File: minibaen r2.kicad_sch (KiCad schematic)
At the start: 131 parts, among them J1 USB_C_Receptacle_USB2.0, Q1 2N7002, SW1 MX_SW_solder, SW10 MX_SW_solder, SW11 MX_SW_solder, SW12 MX_SW_solder, SW13 MX_SW_solder, SW14 MX_SW_solder, SW15 MX_SW_solder, SW16 MX_SW_solder, SW17 MX_SW_solder, SW18 MX_SW_solder, SW19 MX_SW_solder, SW2 MX_SW_solder, SW20 MX_SW_solder, SW21 MX_SW_solder, SW22 MX_SW_solder, SW23 MX_SW_solder, SW24 MX_SW_solder, SW25 MX_SW_solder, SW26 MX_SW_solder, SW27 MX_SW_solder, SW28 MX_SW_solder, SW29 MX_SW_solder, SW3 MX_SW_solder, SW30 MX_SW_solder, SW31 MX_SW_solder, SW32 MX_SW_solder, SW33 MX_SW_solder, SW34 MX_SW_solder, SW35 MX_SW_solder, SW36 MX_SW_solder, SW37 MX_SW_solder, SW38 MX_SW_solder, SW39 MX_SW_solder, SW4 MX_SW_solder, SW40 MX_SW_solder, SW41 MX_SW_solder, SW42 MX_SW_solder, SW43 MX_SW_solder, SW44 MX_SW_solder, SW45 MX_SW_solder, SW46 SW_Push, SW47 MX_SW_solder, SW48 MX_SW_solder, SW49 MX_SW_solder, SW5 MX_SW_solder, SW51 MX_SW_solder, SW52 MX_SW_solder, SW53 MX_SW_solder, SW54 MX_SW_solder, SW6 MX_SW_solder, SW7 MX_SW_solder, SW8 MX_SW_solder, SW9 MX_SW_solder, U3 SRV05-4, U4 XC6206PxxxMR, U5 STM32F072C8Tx

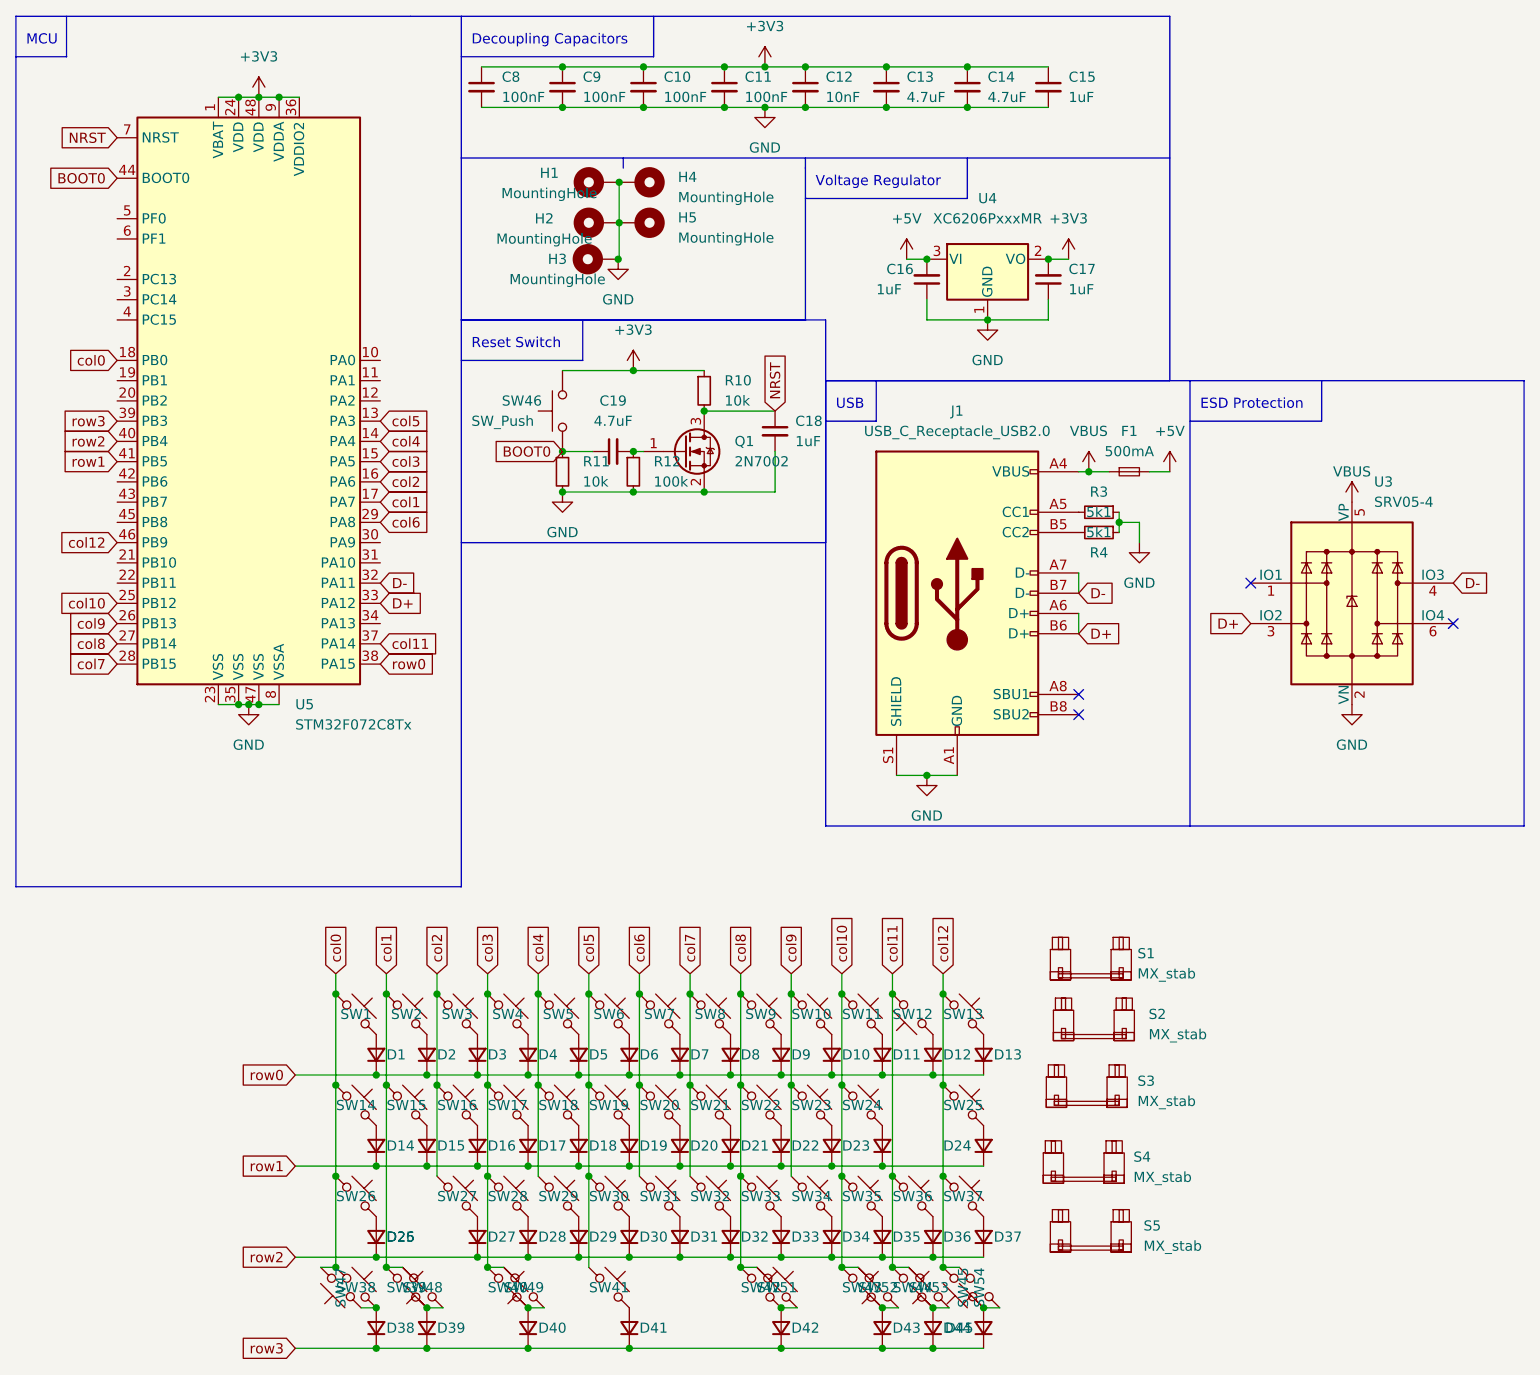
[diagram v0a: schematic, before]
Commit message: updates
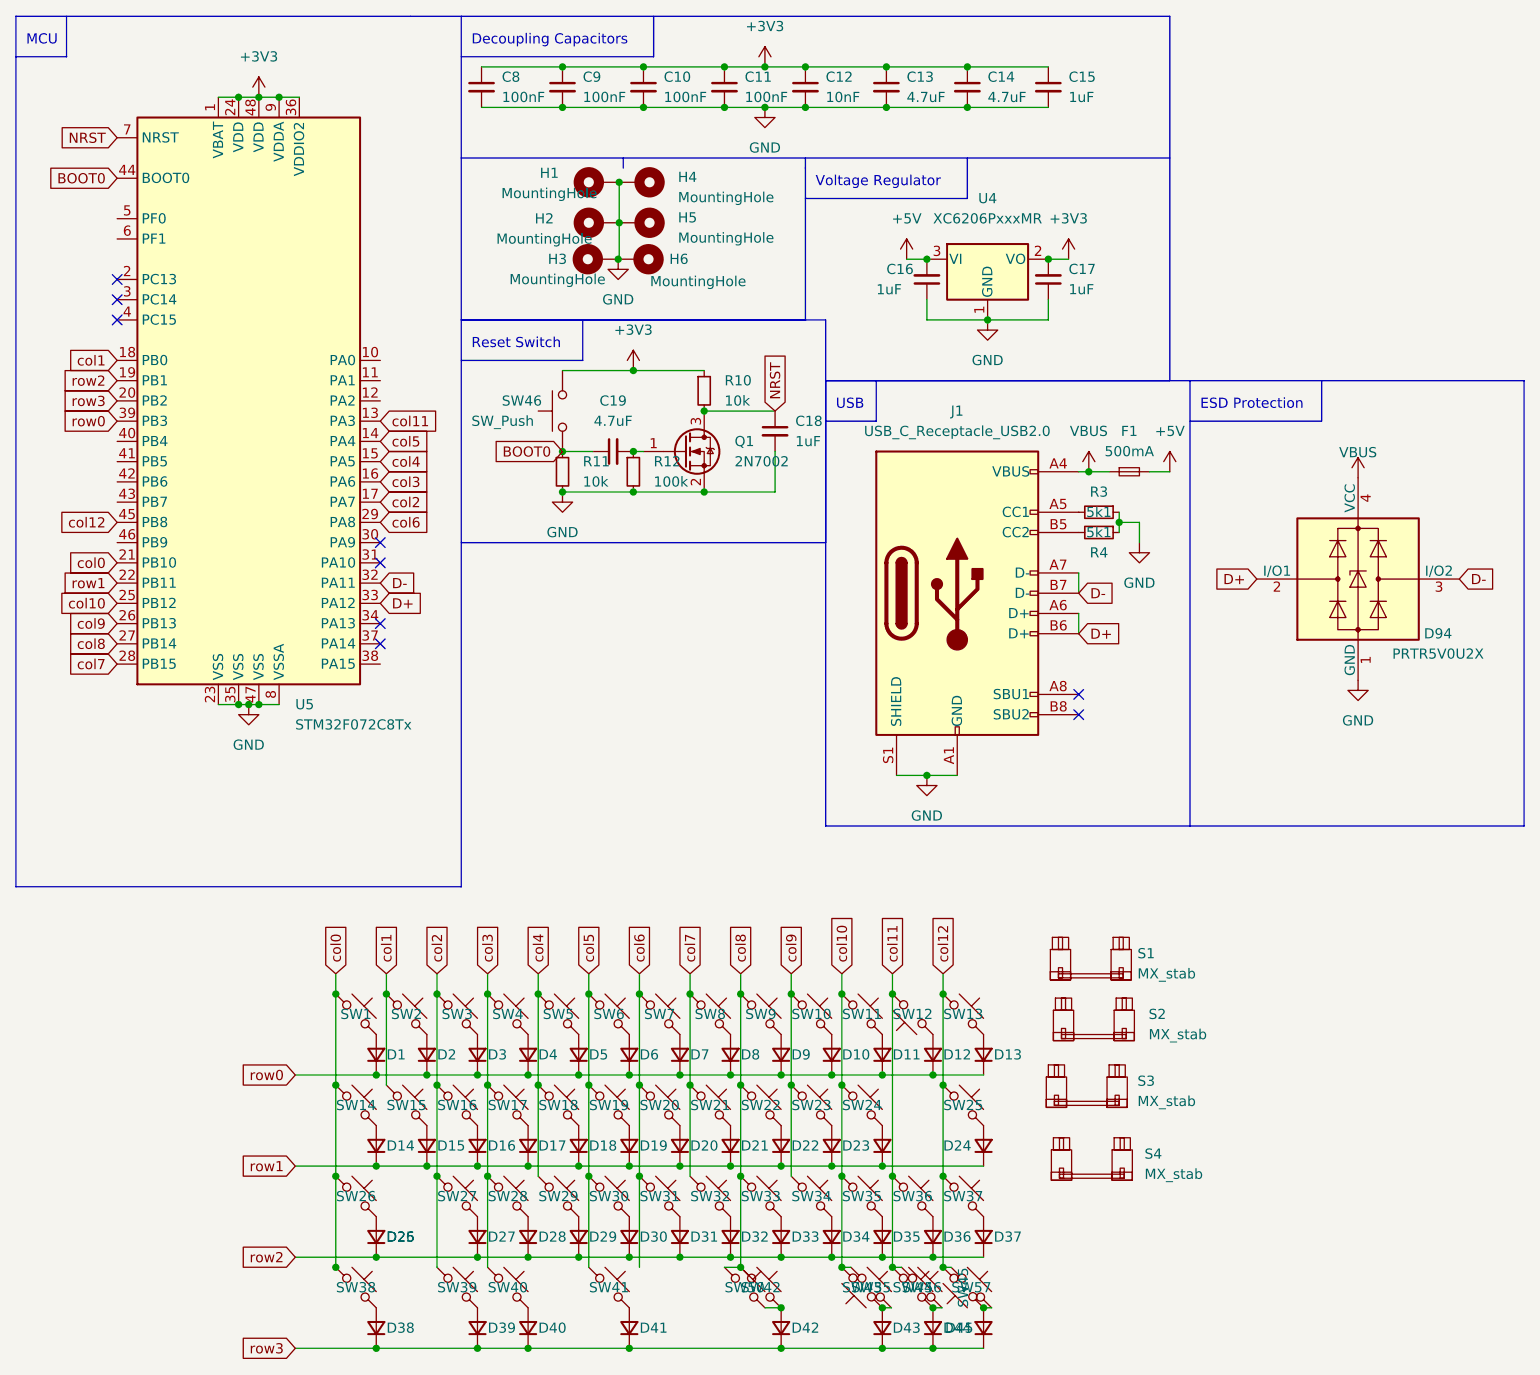
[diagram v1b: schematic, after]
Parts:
- removed S5: MX_stab, marbastlib-mx:STAB_MX_2u, symbol marbastlib-mx:MX_stab
- removed SW47, SW49, SW52, SW54: MX_SW_solder, marbastlib-mx:SW_MX_1.5u, symbol marbastlib-mx:MX_SW_solder
- removed SW48, SW51, SW53: MX_SW_solder, marbastlib-mx:SW_MX_1u, symbol marbastlib-mx:MX_SW_solder
- removed U3: SRV05-4, marbastlib-various:SOT-23-6-routable, symbol Power_Protection:SRV05-4
- added D94: PRTR5V0U2X, Package_TO_SOT_SMD:SOT-143, symbol Power_Protection:PRTR5V0U2X
- added H6: MountingHole, MountingHole:MountingHole_2.2mm_M2_DIN965_Pad, symbol Mechanical:MountingHole_Pad
- added SW50, SW55, SW56, SW57: MX_SW_solder, marbastlib-mx:SW_MX_1u, symbol marbastlib-mx:MX_SW_solder
- S4: footprint marbastlib-mx:STAB_MX_2.75u -> marbastlib-mx:STAB_MX_6.25u
- SW37: footprint marbastlib-mx:SW_MX_1.25u -> marbastlib-mx:SW_MX_1u
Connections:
- net D+: now also D94.2 (I/O1)
- net D-: now also D94.3 (I/O2)
- net GND: now also D94.1 (GND), H6.1
- net VBUS: now also D94.4 (VCC)
- net col0: now also U5.21 (PB10); no longer U5.18 (PB0)
- net col1: now also U5.18 (PB0); no longer SW39.1, U5.17 (PA7)
- net col10: now also SW43.2, SW55.1; no longer SW43.1
- net col11: now also U5.13 (PA3), SW56.1; no longer U5.37 (PA14)
- net col12: now also U5.45 (PB8), SW57.1; no longer U5.46 (PB9)
- net col2: now also SW39.1, U5.17 (PA7); no longer U5.16 (PA6)
- net col3: now also U5.16 (PA6); no longer U5.15 (PA5)
- net col4: now also U5.15 (PA5); no longer U5.14 (PA4)
- net col5: now also U5.14 (PA4); no longer U5.13 (PA3)
- net col8: now also SW50.1
- net row0: now also U5.39 (PB3); no longer U5.38 (PA15)
- net row1: now also U5.22 (PB11); no longer U5.41 (PB5)
- net row2: now also U5.19 (PB1); no longer U5.40 (PB4)
- net row3: now also U5.20 (PB2); no longer U5.39 (PB3)
- net at D45.2 (A), SW45.2: now also SW57.2
- net at D42.2 (A), SW42.2: now also SW50.2
- net at D44.2 (A), SW44.2: now also SW56.2
- net at D43.2 (A): now also SW43.1, SW55.2; no longer SW43.2
- no-connect marks 4 -> 9
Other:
- moved on the sheet: D39, SW39, SW43

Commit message: idk
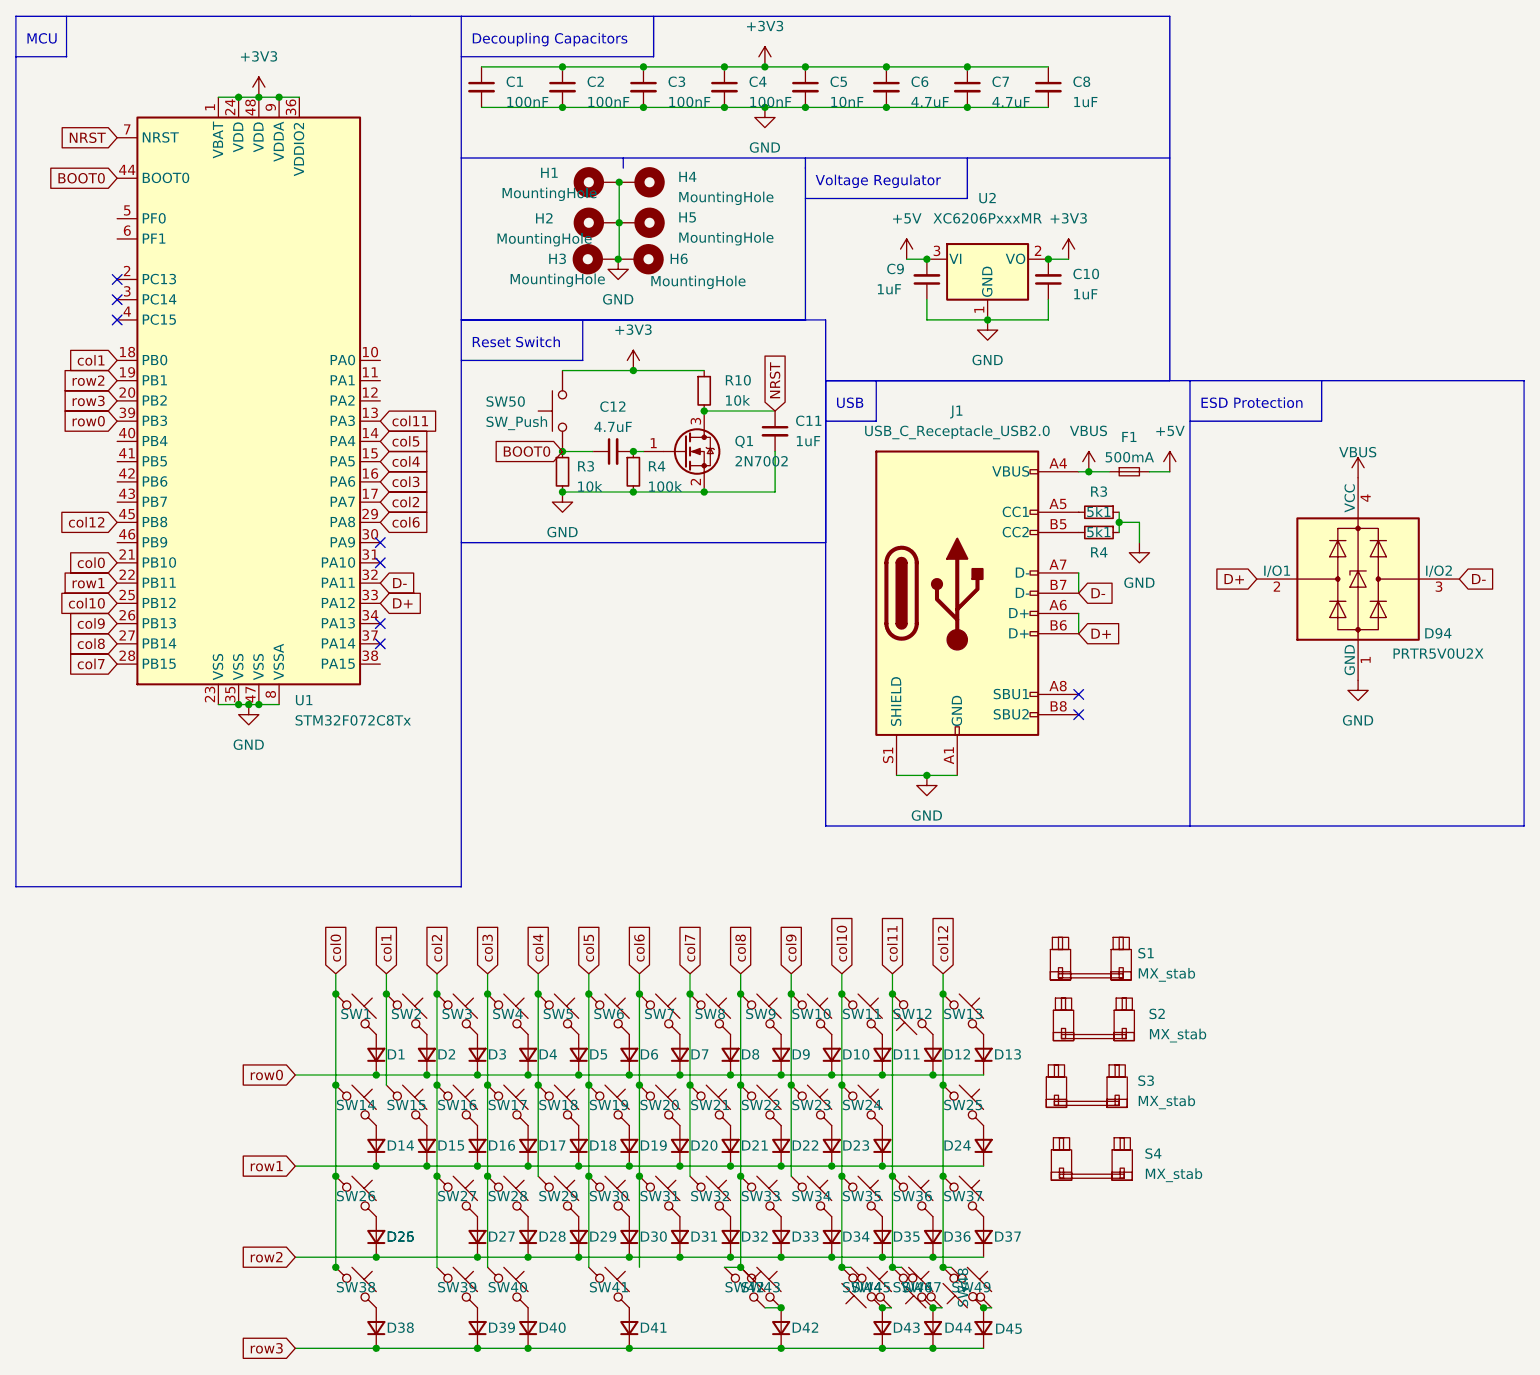
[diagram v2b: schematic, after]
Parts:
- removed SW46: SW_Push, Button_Switch_SMD:SW_SPST_TL3342, symbol Switch:SW_Push
- removed SW50, SW55, SW56, SW57: MX_SW_solder, marbastlib-mx:SW_MX_1u, symbol marbastlib-mx:MX_SW_solder
- added SW46, SW47, SW49: MX_SW_solder, marbastlib-mx:SW_MX_1u, symbol marbastlib-mx:MX_SW_solder
- added SW48: MX_SW_solder, marbastlib-mx:SW_MX_1.25u, symbol marbastlib-mx:MX_SW_solder
- added SW50: SW_Push, Button_Switch_SMD:SW_SPST_TL3342, symbol Switch:SW_Push
- SW43, SW45: footprint marbastlib-mx:SW_MX_1.25u -> marbastlib-mx:SW_MX_1u
- SW44: footprint marbastlib-mx:SW_MX_1u -> marbastlib-mx:SW_MX_1.25u
- renumbered C8 to C1, C17 to C10, C18 to C11, C19 to C12, C9 to C2, C10 to C3, C11 to C4, C12 to C5, C13 to C6, C14 to C7, C15 to C8, C16 to C9, R11 to R3, R12 to R4, U5 to U1, U4 to U2
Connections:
- net +3V3: now also SW50.2
- net BOOT0: now also SW50.1
- net col10: now also SW44.2, SW45.1; no longer SW43.2
- net col11: now also SW46.1, SW47.2; no longer SW44.1
- net col12: now also SW48.1, SW49.1; no longer SW45.1
- net col8: now also SW43.1
- net at D45.2 (A): now also SW48.2, SW49.2; no longer SW45.2
- net at D42.2 (A), SW42.2: now also SW43.2
- net at D44.2 (A): now also SW46.2, SW47.1; no longer SW44.2
- net at D43.2 (A): now also SW44.1, SW45.2; no longer SW43.1
